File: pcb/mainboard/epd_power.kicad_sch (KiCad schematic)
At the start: 79 parts, among them Q1 AO3401A, Q2 S8050, Q6 AO3400A, Q7 AO3401A, Q8 AO3401A, U11 LM321, U23 LGS6302B5, U24 LGS6302B5, U26 LGS5145, U6 MT9700, U7 TPS22914BYFPR, U8 TPS22914BYFPR, U9 LGS5145

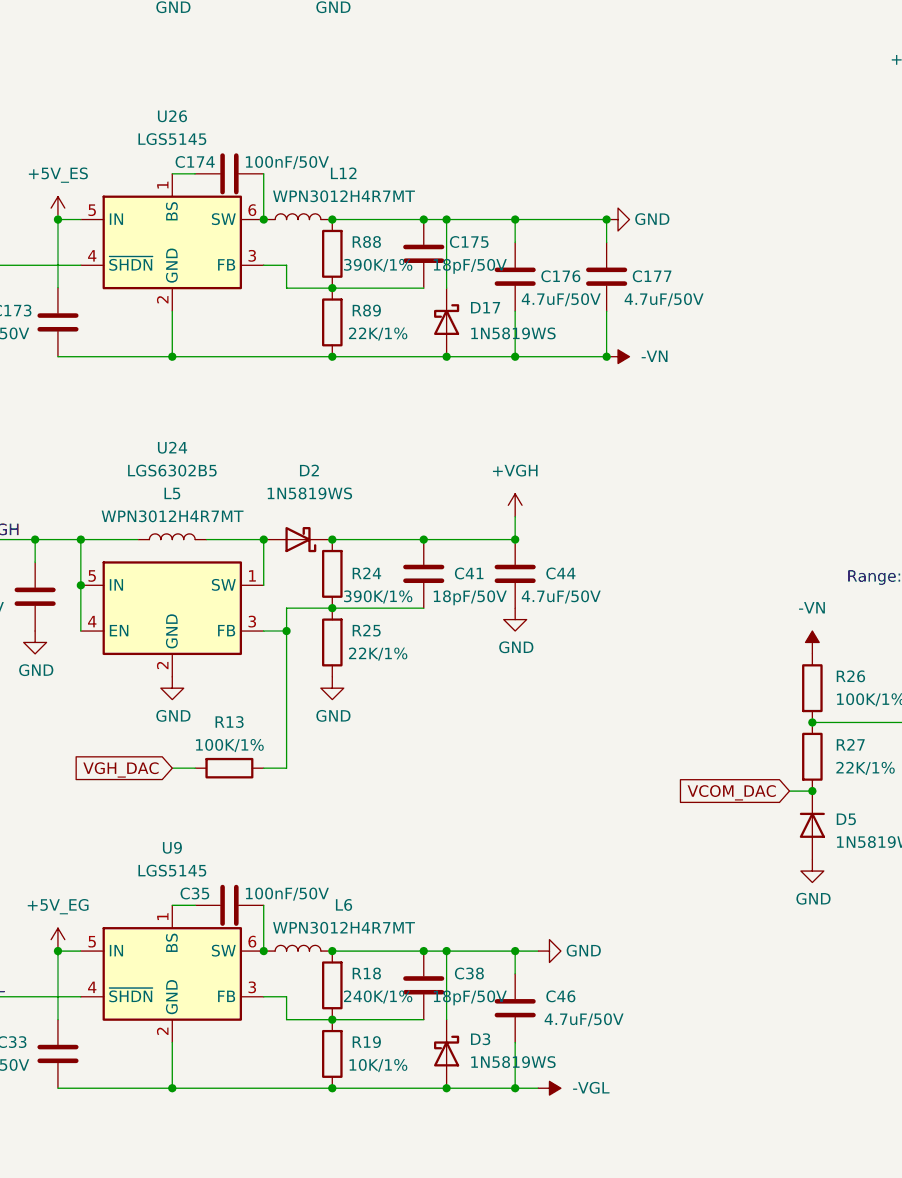
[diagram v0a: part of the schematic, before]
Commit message: PCB r1p3
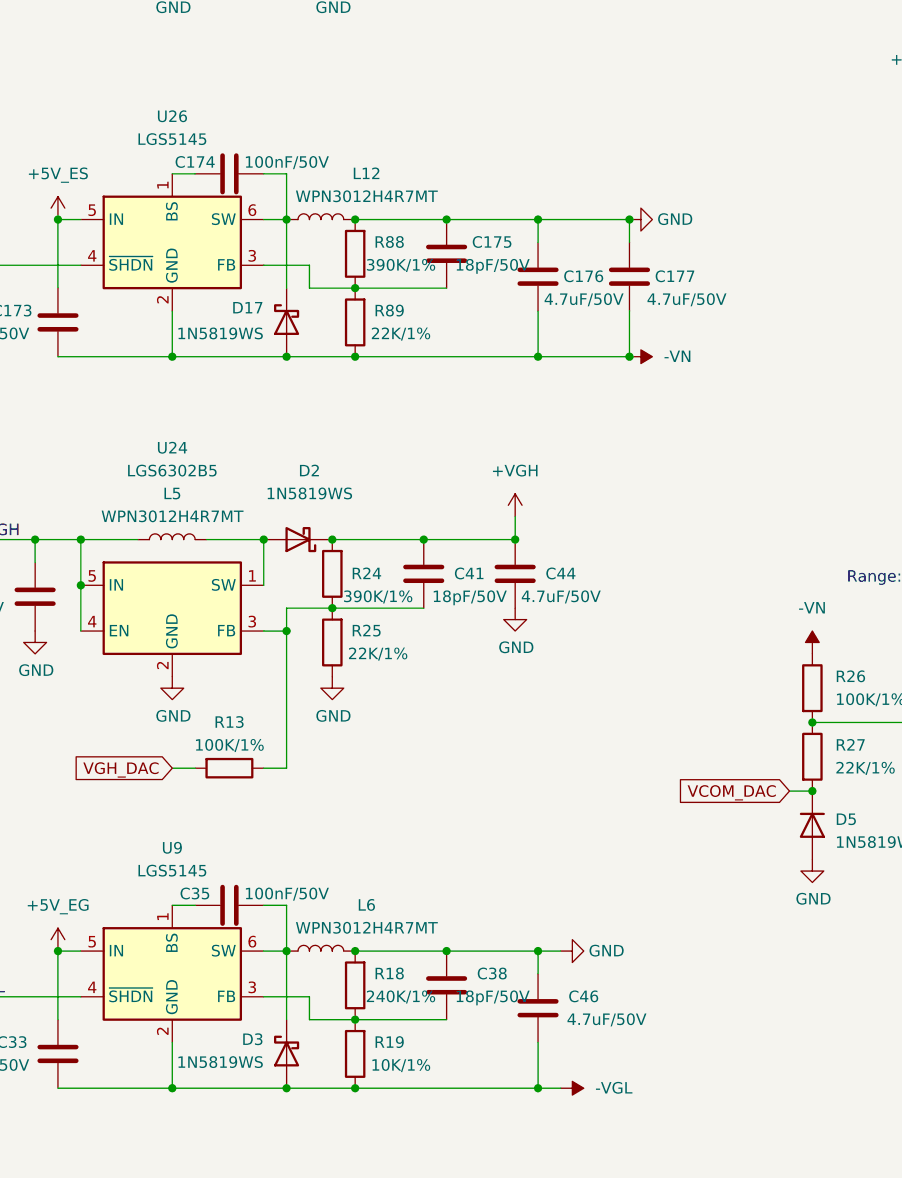
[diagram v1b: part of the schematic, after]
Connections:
- net GND: no longer D17.1 (K), D3.1 (K)
- net at C35.1, L6.1, U9.6 (SW): now also D3.1 (K)
- net at C174.1, L12.1, U26.6 (SW): now also D17.1 (K)
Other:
- moved on the sheet: C175, C176, C177, C38, C46, D17, D3, L12, L6, R18, R19, R88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

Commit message: Sync local PCB changes
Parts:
- U7, U8: footprint Package_CSP:WLCSP-4-X1-WLB0909-4_0.89x0.89mm_P0.5mm -> Package_BGA:WLP-4_0.83x0.83mm_P0.4mm
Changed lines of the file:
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@@
 			)
 		)
-		(property "Footprint" "Package_CSP:WLCSP-4-X1-WLB0909-4_0.89x0.89mm_P0.5mm"
+		(property "Footprint" "Package_BGA:WLP-4_0.83x0.83mm_P0.4mm"
 			(at 82.55 120.65 0)
 			(effects
@@
 			)
 		)
-		(property "Footprint" "Package_CSP:WLCSP-4-X1-WLB0909-4_0.89x0.89mm_P0.5mm"
+		(property "Footprint" "Package_BGA:WLP-4_0.83x0.83mm_P0.4mm"
 			(at 82.55 41.91 0)
 			(effects
